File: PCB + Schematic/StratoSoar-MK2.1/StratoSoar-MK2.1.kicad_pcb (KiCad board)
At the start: 4 copper layers, 42 x 87.9 mm, 110 parts, among them J1 BME280, J10 parachute, J11 VOUT, J12 VIN, J2 AT_ISP, J3 AT_FTDI, J4 Signal, J5 USB_C_Receptacle_USB2.0, J6 JTAG, J7 Power, J8 rudder, J9 elevator, Q1 2N3906, Q2 2N3906, Q3 2N3906, Q4 DMN1019USN-13, Q5 DMN1019USN-13, Q6 DMN1019USN-13, SW1 AT_RESET, SW2 EEPROM, SW3 AAA, SW4 PWR_SW, SW5 RESET, U1 MAX-M10S, U2 MPU-9250, U3 ATmega328P-A, U4 AT24C512C-SSHD-T, U5 ATXK-H11-E-32.768KHZ-E50-T3, U6 ATSAMD21G18A-A, U7 MCP1700x-330xxTT, Y1 8MHz, Y2 32.768kHz

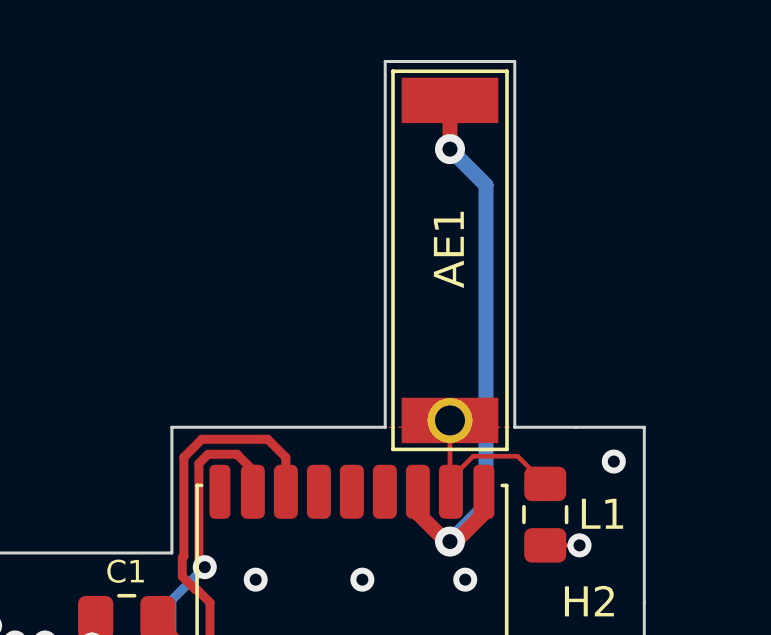
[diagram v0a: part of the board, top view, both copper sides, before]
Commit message: Test
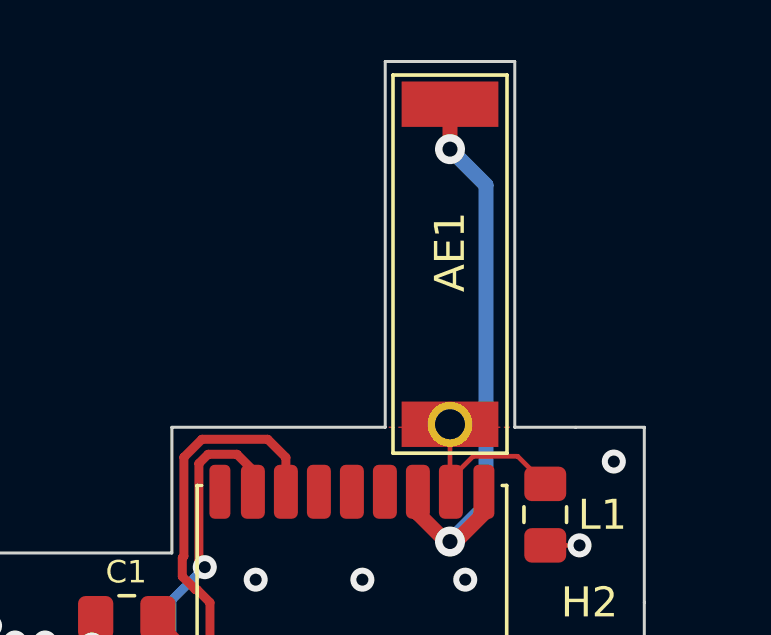
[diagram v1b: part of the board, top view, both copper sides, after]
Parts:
- moved AE1 0.13 mm to (87.2, 30.7)
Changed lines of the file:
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@@
 	(footprint "RF_Antenna:RAINSUN_GPS1003"
 		(layer "F.Cu")
-		(at 87.249 30.6086 -90)
+		(at 87.249 30.7356 -90)
 		(descr "RFID Transponder Coil")
 		(tags "antenna rfid coilcraft")

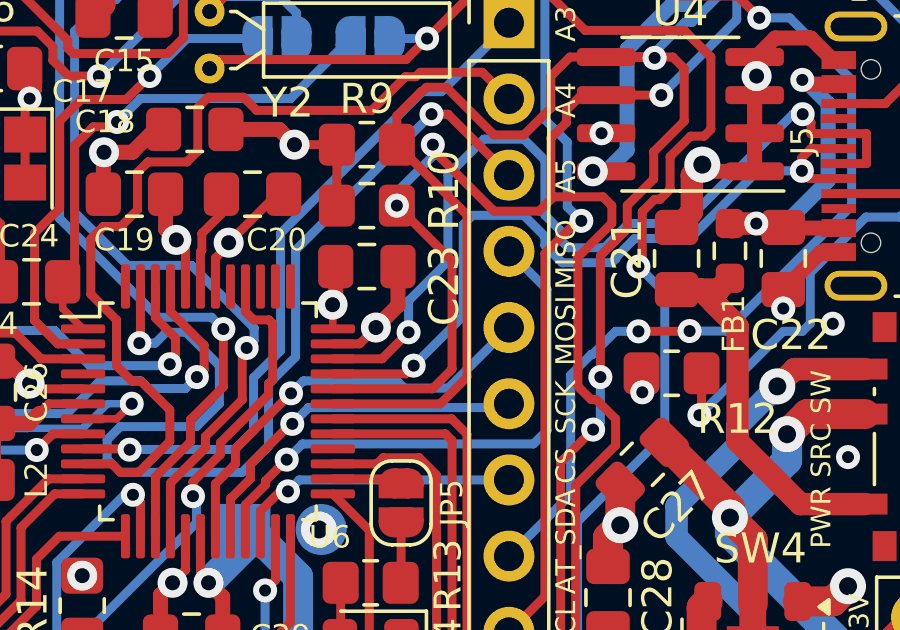
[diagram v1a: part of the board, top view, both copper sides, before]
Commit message: Update
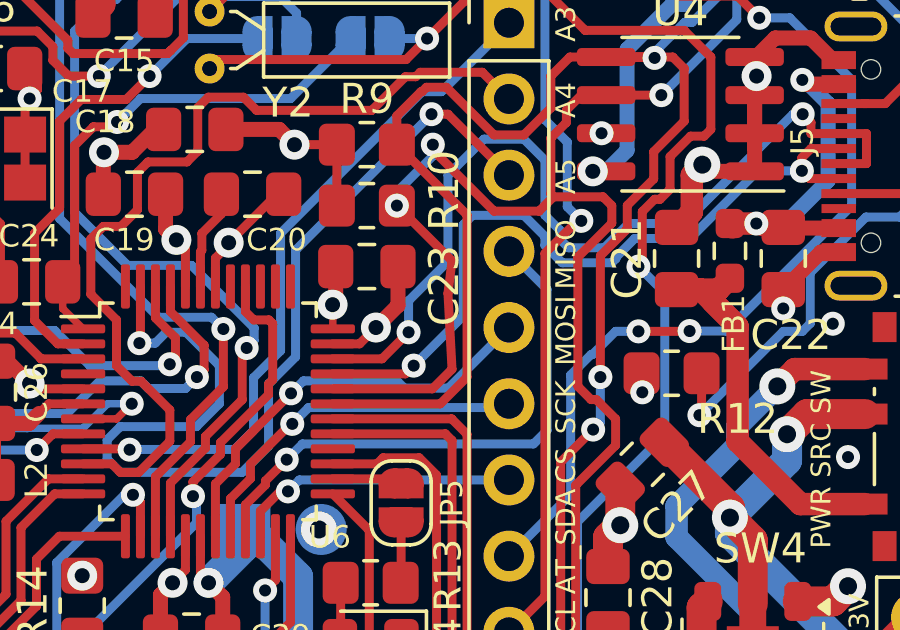
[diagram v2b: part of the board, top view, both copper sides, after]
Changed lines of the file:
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@@
+	)
+	(segment
+		(start 75.946 78.74)
+		(end 76.081 81.272)
+		(width 0.3)
+		(layer "F.Cu")
+		(net 42)
 	)
 	(segment
@@
 	)
 	(segment
+		(start 76.081 77.658)
+		(end 75.946 78.74)
+		(width 0.3)
+		(layer "F.Cu")
+		(net 42)
+	)
+	(segment
 		(start 80.715339 82.284)
 		(end 80.276 81.844661)
@@
 		(width 0.3)
 		(layer "F.Cu")
-		(net 42)
-	)
-	(segment
-		(start 76.081 77.658)
-		(end 76.081 81.272)
-		(width 0.3)
-		(layer "F.Cu")
